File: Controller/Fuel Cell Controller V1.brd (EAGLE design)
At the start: 100 x 80 mm, 8 parts

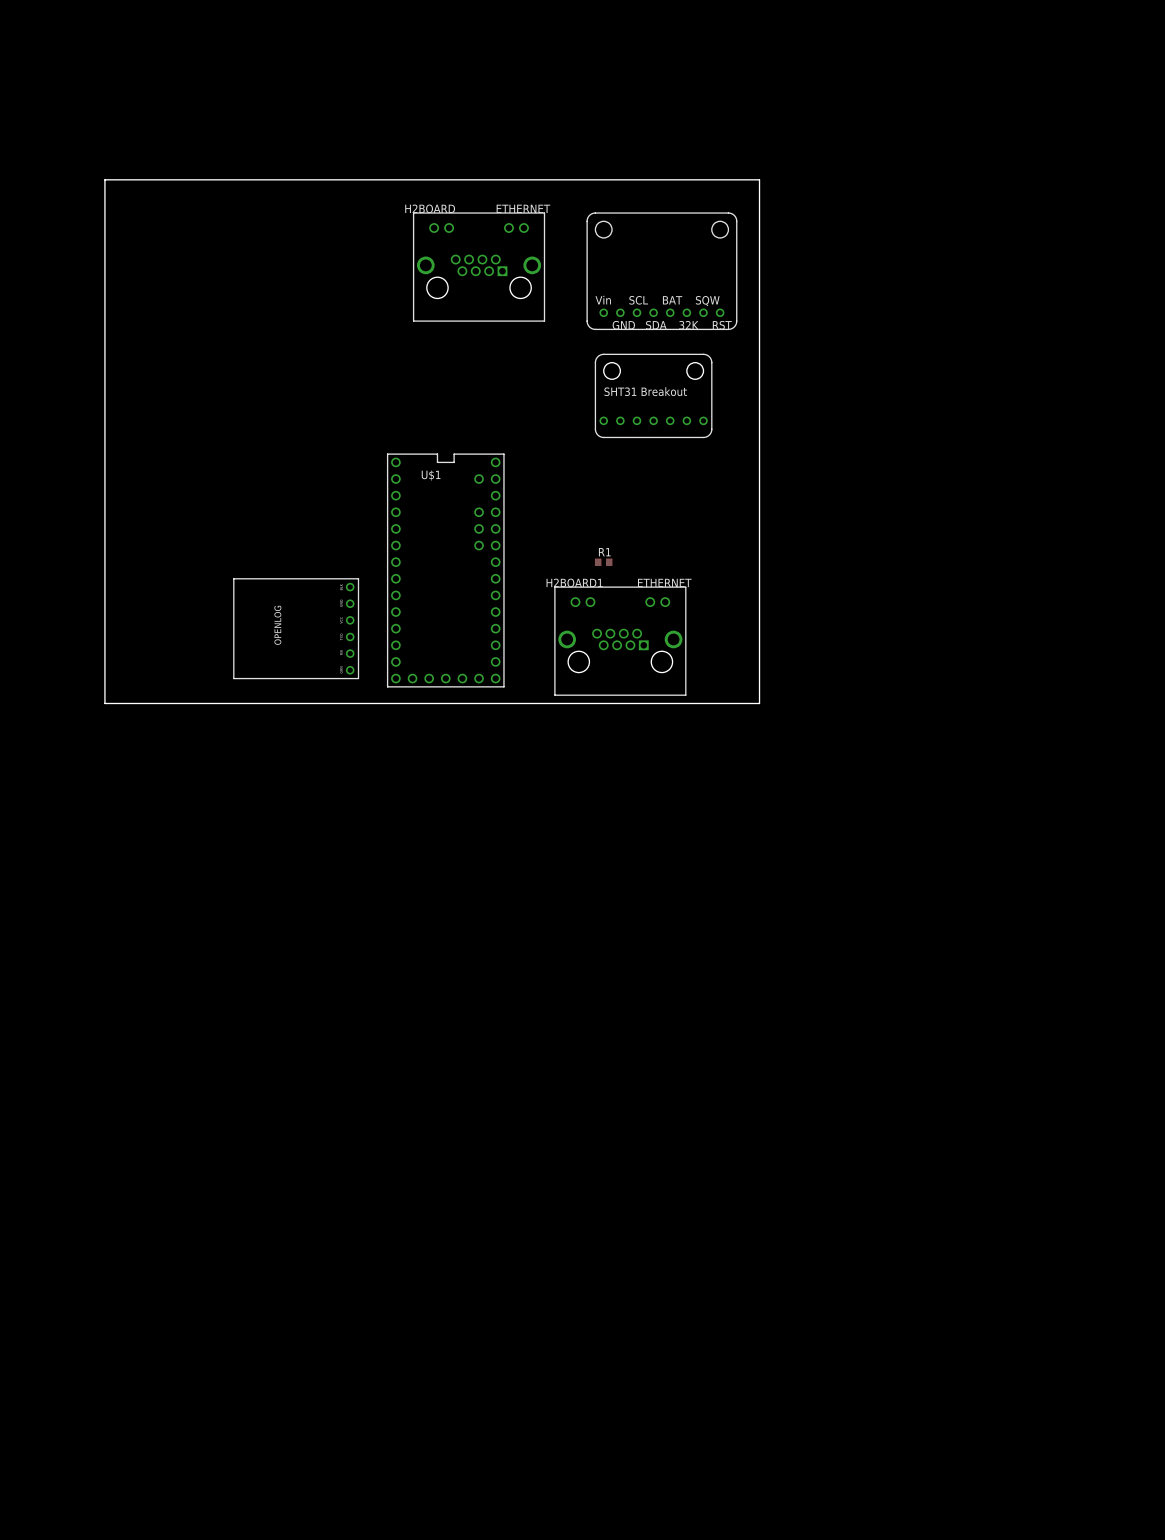
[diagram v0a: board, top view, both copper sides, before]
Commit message: update
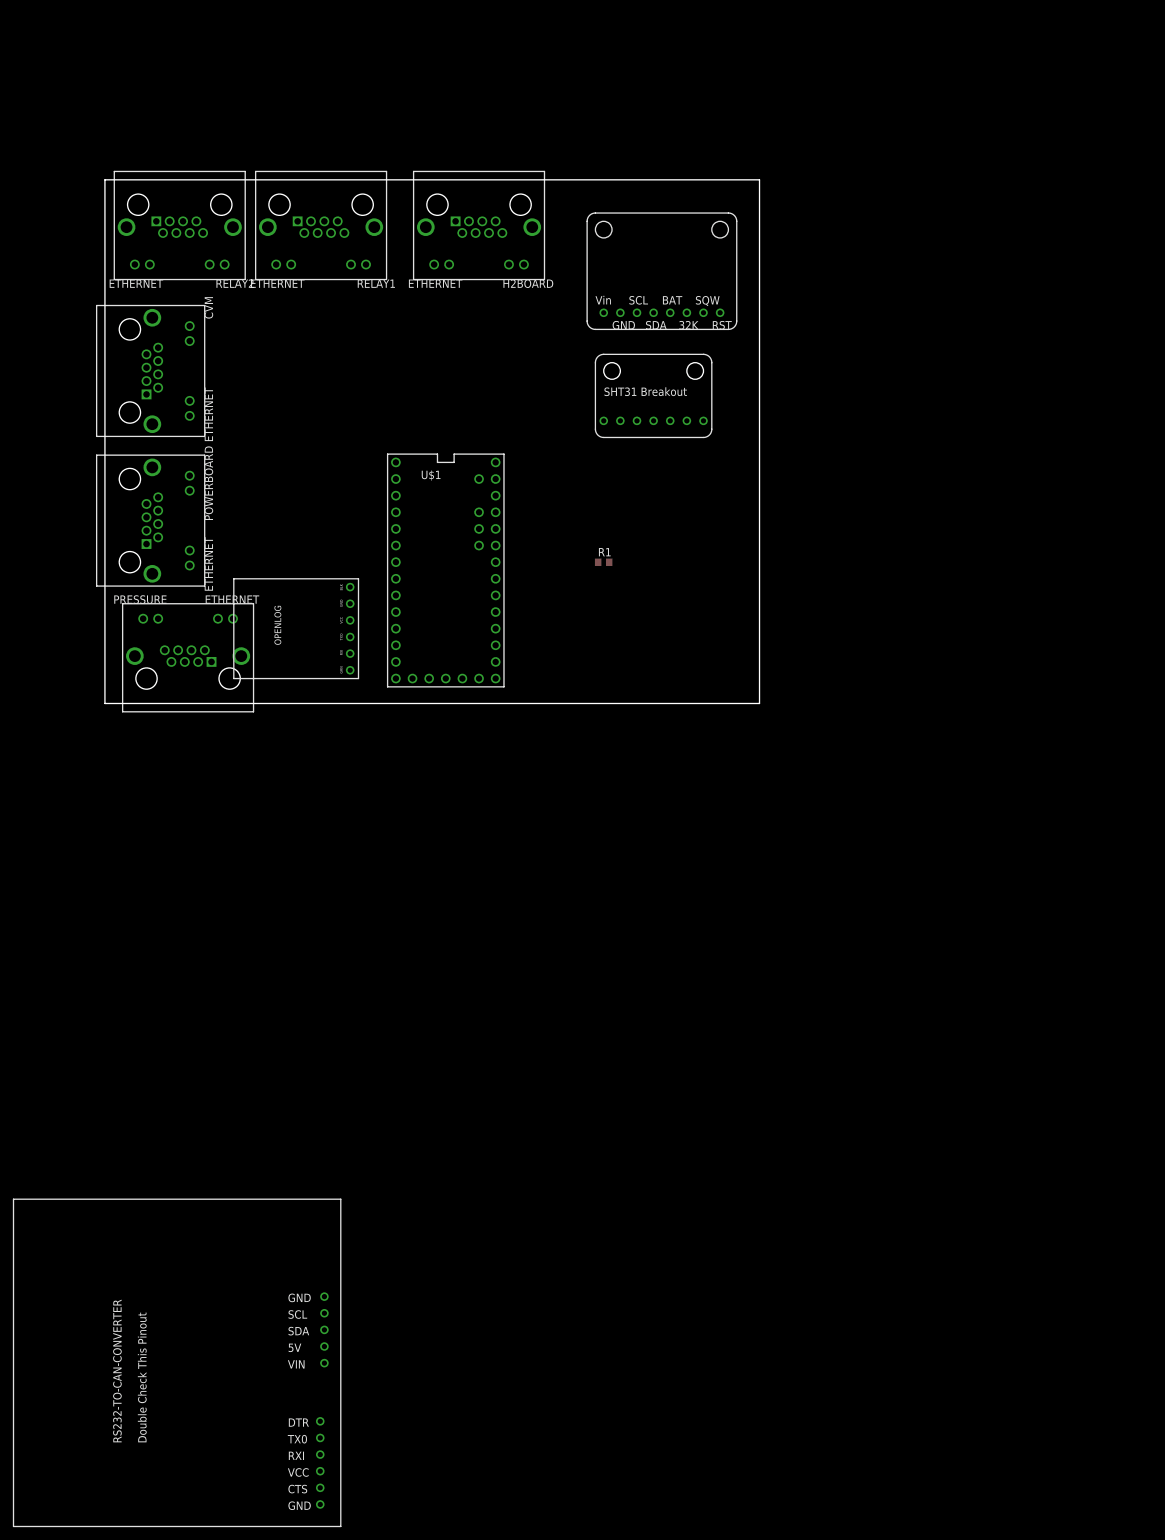
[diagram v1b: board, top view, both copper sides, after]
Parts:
- removed H2BOARD1: ETHERNET, ETHERNET:A122645-ND
- added CVM, POWERBOARD, PRESSURE, RELAY1, RELAY2: ETHERNET, ETHERNET:A122645-ND
- added FRAME2: FRAME-LETTERNO_PACKAGE, SparkFun-Aesthetics:DUMMY
- added U$5: RS232-TO-CAN-CONVERTER, rs232-to-can:RS232-TO-CAN-CONVERTER
- moved H2BOARD 12.7 mm to (57.1, 76.2), turned to 180 degrees
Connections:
- removed net 12V_AUX: H2BOARD.P$6
- removed net FC_R: H2BOARD1.P$6
- removed net MISO: U$1.12
- removed net MOSI: U$1.11
- removed net SCK: U$1.13
- new net AUX12: H2BOARD.P$6, POWERBOARD.P$3, RELAY1.P$5
- new net CAP_R: RELAY1.P$3, U$1.11
- new net CHARGE_R: RELAY1.P$4, U$1.12
- new net EXTRA_V: U$1.10
- new net FC12: POWERBOARD.P$1, POWERBOARD.P$2, PRESSURE.P$1, RELAY1.P$6
- new net FCC_R: POWERBOARD.P$8, RELAY2.P$6, U$1.20/A6
- new net FCPRES: PRESSURE.P$3, U$1.23/A9
- new net MOTOR_R: RELAY1.P$2, U$1.22/A8
- new net N$1: CVM.P$1
- new net N$2: CVM.P$2
- new net N$3: CVM.P$3
- new net N$4: CVM.P$4
- new net N$5: CVM.P$5
- new net N$6: CVM.P$6
- new net N$7: CVM.P$7
- new net N$8: CVM.P$8
- new net PURGE_V: U$1.9
- new net START_R: RELAY1.P$1, U$1.21/A7
- new net SUPPLY_V: U$1.6
- net 5V: now also POWERBOARD.P$4, RELAY2.P$5, U$5.5V, U$5.VCC; no longer H2BOARD1.P$5
- net CAPCURR: now also RELAY2.P$1; no longer H2BOARD1.P$1
- net CAPVOLT: now also RELAY2.P$3; no longer H2BOARD1.P$3
- net FCCURR: now also RELAY2.P$2; no longer H2BOARD1.P$2
- net FCVOLT: now also RELAY2.P$4; no longer H2BOARD1.P$4
- net GND: now also CVM.P$13, CVM.P$14, POWERBOARD.P$13, POWERBOARD.P$14, POWERBOARD.P$5, POWERBOARD.P$6, POWERBOARD.P$7, PRESSURE.P$2, RELAY1.P$13, RELAY1.P$14, RELAY1.P$7, RELAY1.P$8, RELAY2.P$13, RELAY2.P$14, RELAY2.P$7, RELAY2.P$8, U$5.GND, U$5.GND_; no longer H2BOARD1.P$13, H2BOARD1.P$14, H2BOARD1.P$7, H2BOARD1.P$8
- net RX1: now also U$5.TX0
- net TX1: now also U$5.RXI

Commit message: update
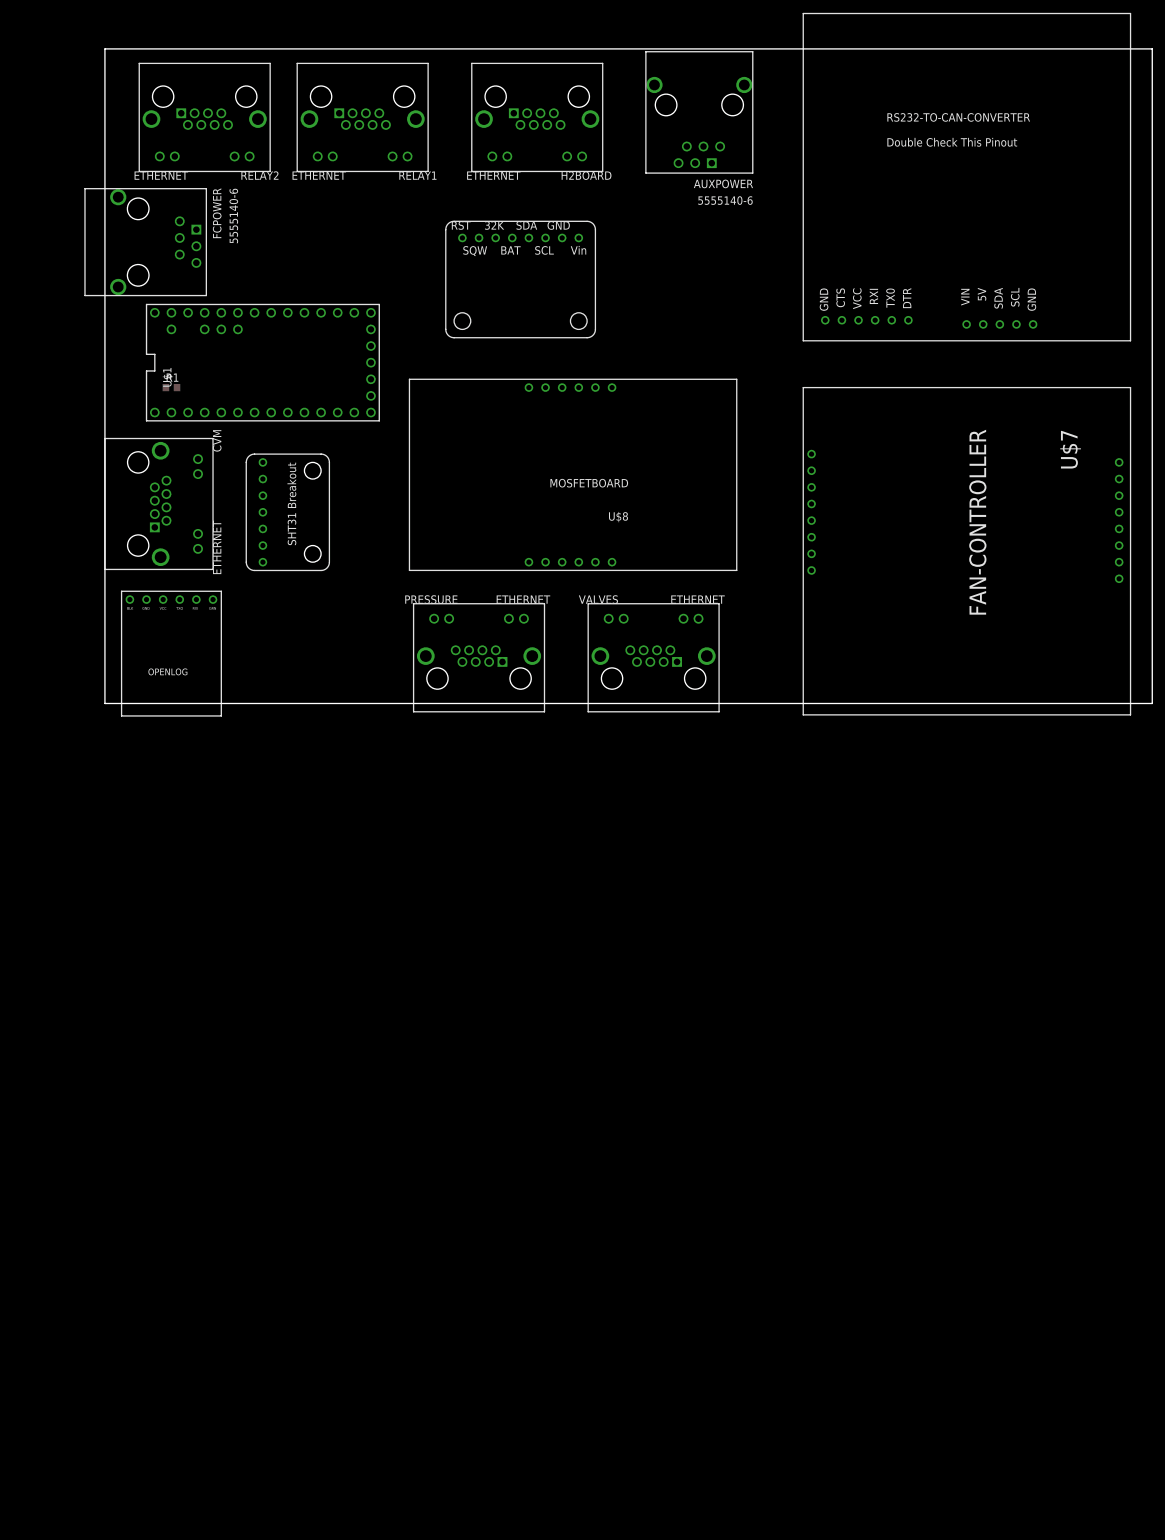
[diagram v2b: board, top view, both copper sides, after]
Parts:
- removed POWERBOARD: ETHERNET, ETHERNET:A122645-ND
- added AUXPOWER, FCPOWER: 5555140-6, 5555140-6 RJ11:1734723-1_RJ11
- added U$7: FAN-CONTROLLER, fan controller:FAN-CONTROLLER
- added U$8: MOSFETBOARD, mosfet board:MOSFET-BOARD
- added VALVES: ETHERNET, ETHERNET:A122645-ND
- moved U$5 260.7 mm to (106.7, 105.4), turned to 270 degrees
- moved R1 71.2 mm to (10.2, 48.3)
- moved U$3 53.4 mm to (21.6, 38.1), turned to 270 degrees
- moved PRESSURE 44.5 mm to (57.1, 3.81)
- moved U$1 42.3 mm to (24.1, 52.1), turned to 90 degrees
- moved CVM 20.4 mm to (5.08, 30.5)
- moved U$2 19.4 mm to (10.2, 7.62), turned to 180 degrees
- moved H2BOARD 18.8 mm to (66.0, 92.7)
- moved RELAY1 17.7 mm to (39.4, 92.7)
- moved RELAY2 16.9 mm to (15.2, 92.7)
- moved U$4 16.6 mm to (74.9, 73.7), turned to 180 degrees
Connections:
- removed net +5V: U$1.VIN
- new net AUX5: AUXPOWER.3, AUXPOWER.4, H2BOARD.P$8, U$5.5V, U$5.VCC
- new net EXTRA_V_G: U$8.OUT3, VALVES.P$6
- new net FC5: FCPOWER.3, FCPOWER.4, U$1.VIN, U$2.P$4, U$7.5, U$7.5_2, U$8.VDD
- new net N$16: PRESSURE.P$4
- new net N$17: PRESSURE.P$5
- new net N$18: PRESSURE.P$6
- new net N$19: PRESSURE.P$7
- new net N$20: PRESSURE.P$8
- new net N$21: PRESSURE.P$13
- new net N$22: PRESSURE.P$14
- new net PURGE_V_G: U$8.OUT2, VALVES.P$4
- new net SUPPLY_V_G: U$8.OUT1, VALVES.P$2
- net +3.3V: no longer U$2.P$4
- net 5V: no longer H2BOARD.P$8, POWERBOARD.P$4, U$5.5V, U$5.VCC
- net AUX12: now also AUXPOWER.1, AUXPOWER.2, VALVES.P$1; no longer POWERBOARD.P$3
- net EXTRA_V: now also U$8.IN3
- net FC12: now also FCPOWER.1, FCPOWER.2, U$7.12, U$7.12_2, U$7.12_3, VALVES.P$3, VALVES.P$5; no longer POWERBOARD.P$1, POWERBOARD.P$2
- net FCC_R: no longer POWERBOARD.P$8
- net GND: now also AUXPOWER.5, AUXPOWER.6, AUXPOWER.SH1, AUXPOWER.SH2, FCPOWER.5, FCPOWER.6, FCPOWER.SH1, FCPOWER.SH2, U$7.GND, U$7.GND2, U$7.GND3, U$8.GND, U$8.GND1, U$8.GND2, U$8.VSS, VALVES.P$13, VALVES.P$14; no longer POWERBOARD.P$13, POWERBOARD.P$14, POWERBOARD.P$5, POWERBOARD.P$6, POWERBOARD.P$7
- net H2_OK: now also U$8.ESTOP
- net PURGE_V: now also U$8.IN2
- net SCL: now also U$7.SCL
- net SDA: now also U$7.SDA
- net SUPPLY_V: now also U$8.IN1
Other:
- board size 100 x 80 mm -> 160 x 100 mm
